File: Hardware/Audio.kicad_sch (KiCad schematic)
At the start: 16 parts, among them J5 MJ-3536NG, U11 PAM8302AAD, U9 PCM1809

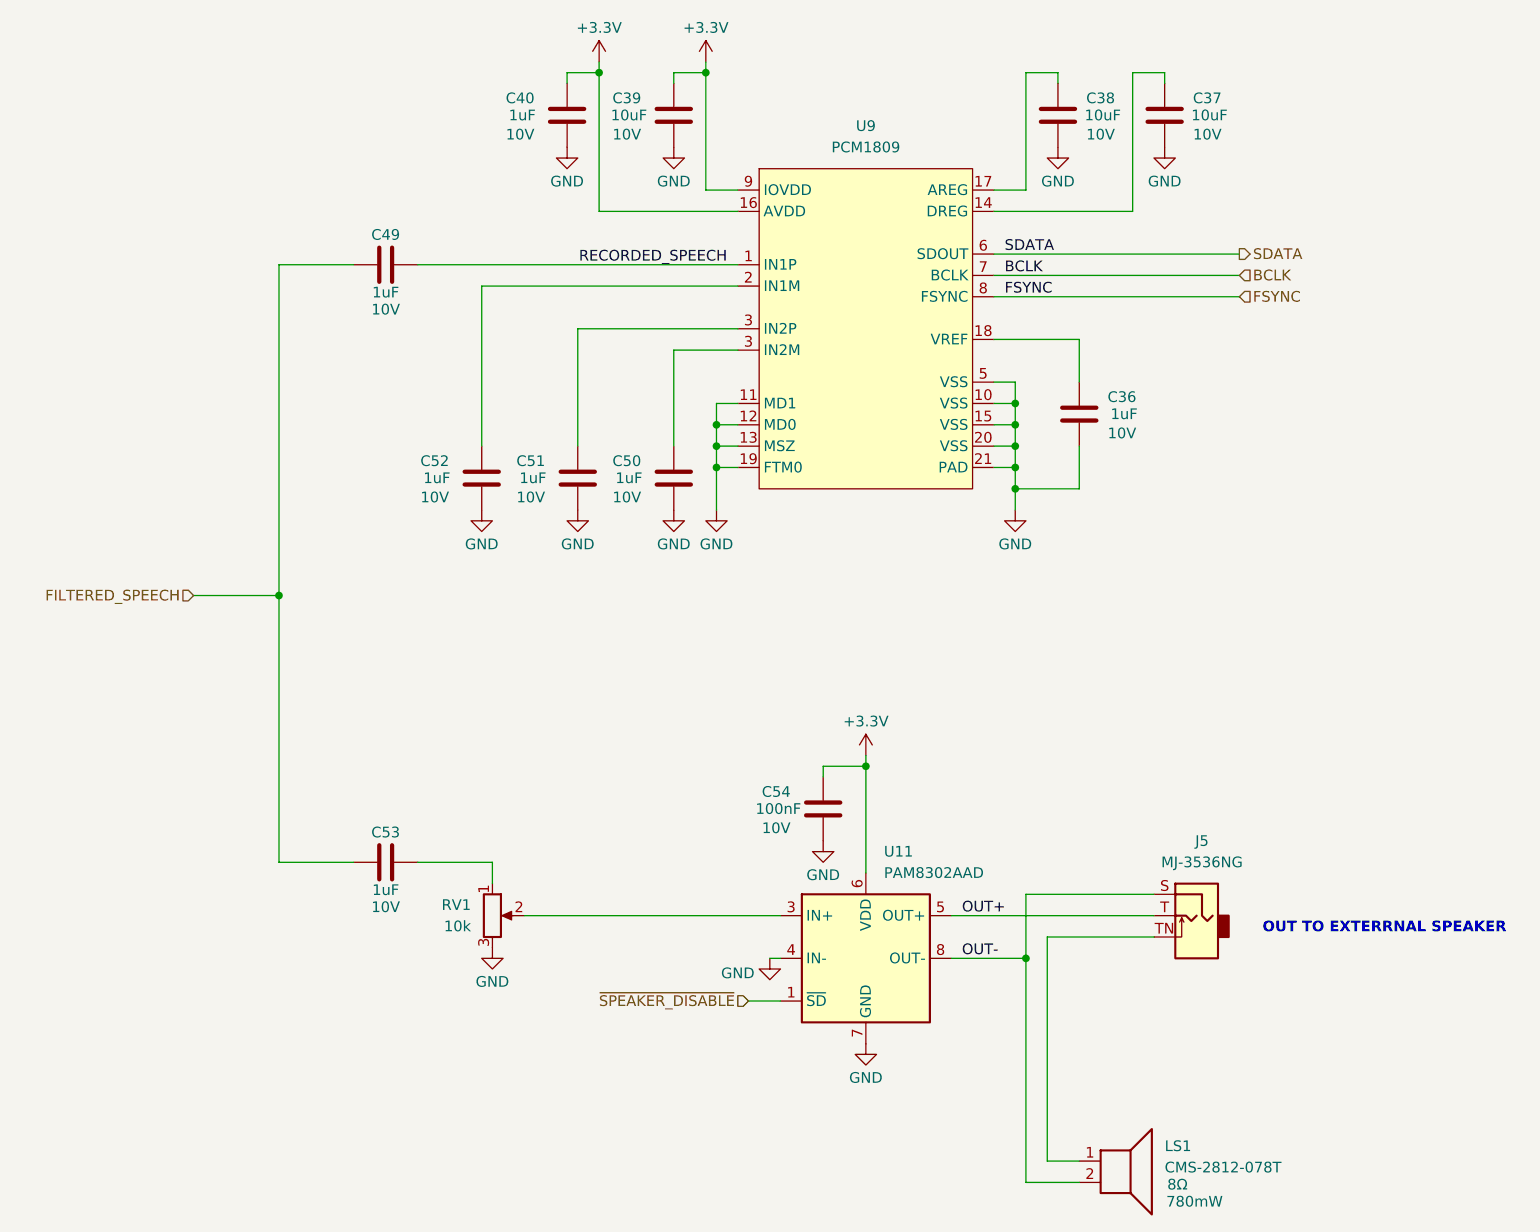
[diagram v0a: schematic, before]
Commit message: finalize audio outputs
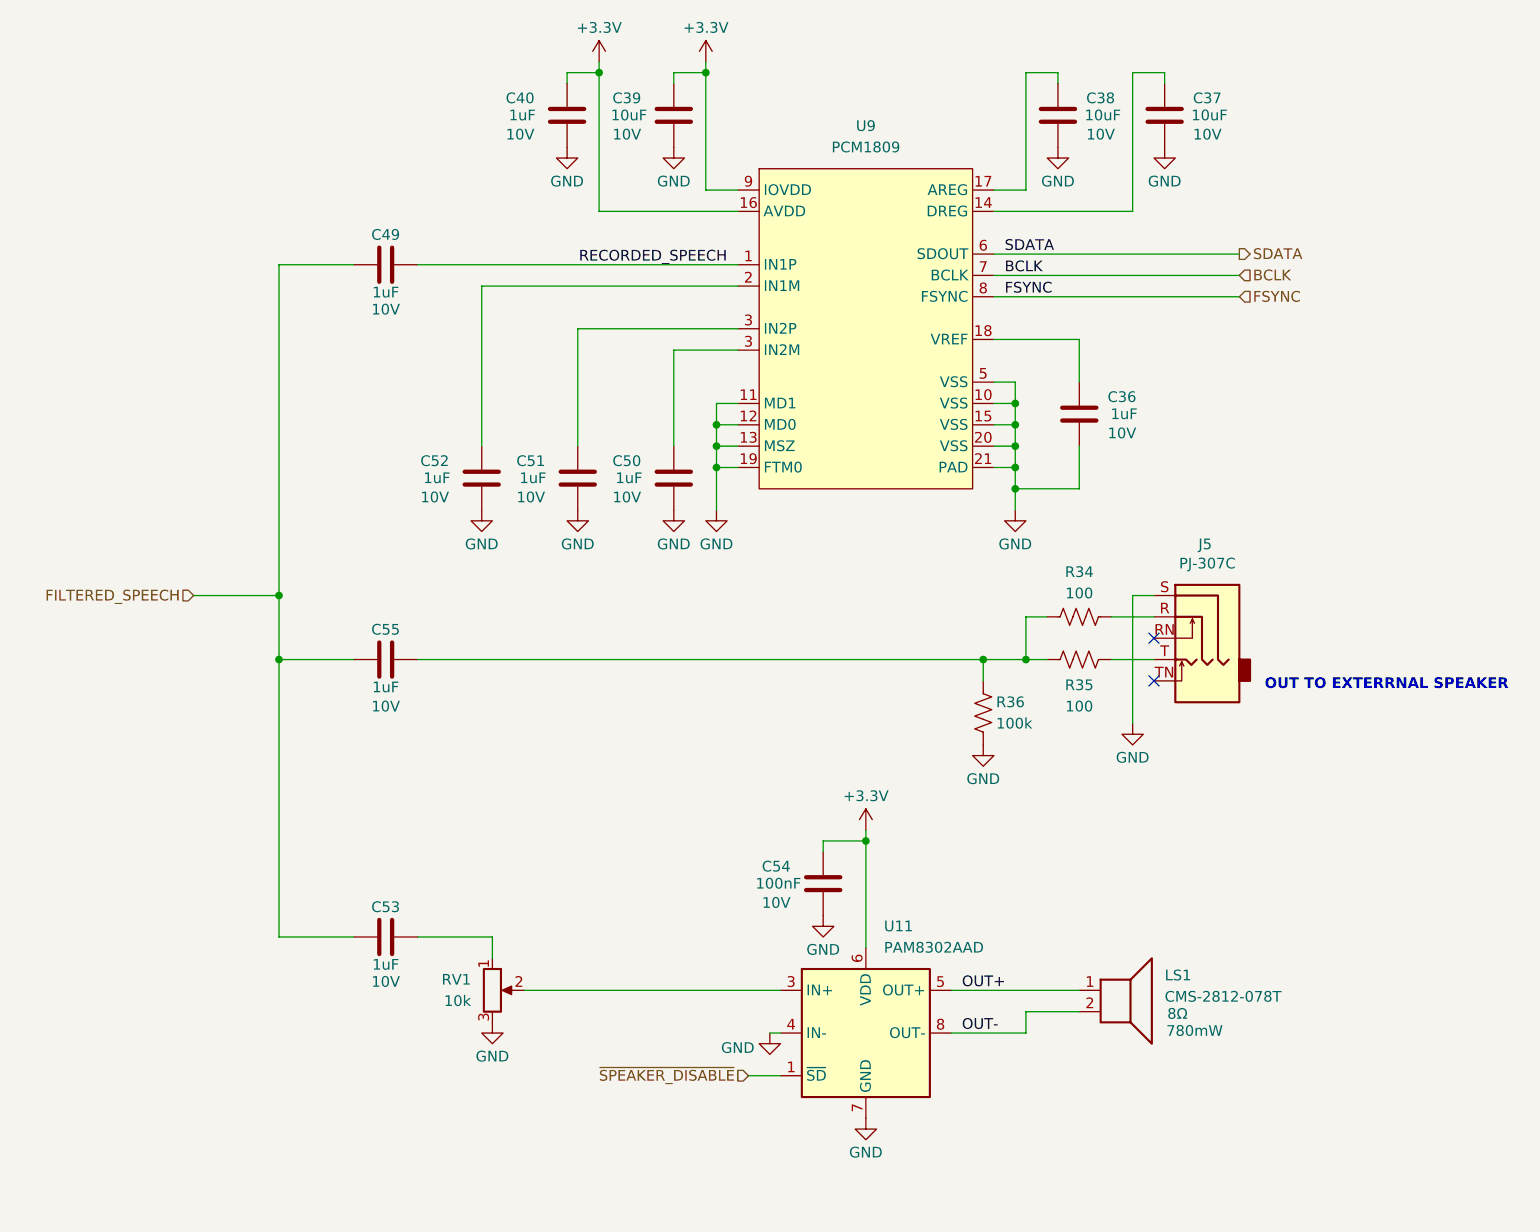
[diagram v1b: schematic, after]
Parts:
- removed J5: MJ-3536NG, symbol Connector_Audio:AudioJack2_SwitchT
- added C55: 1uF, symbol Device:C
- added J5: PJ-307C, symbol Connector_Audio:AudioJack3_SwitchTR
- added R34, R35: 100, symbol Device:R_US
- added R36: 100k, symbol Device:R_US
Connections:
- net FILTERED_SPEECH: now also C55.2
- net GND: now also J5.S, R36.2
- net OUT+: now also LS1.1
- new net: J5.R, R34.1
- new net: C55.1, R34.2, R35.2, R36.1
- new net: J5.T, R35.1
- no-connect marks 0 -> 2
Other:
- moved on the sheet: C53, C54, LS1, RV1, U11
